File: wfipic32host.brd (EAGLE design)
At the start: 95.2 x 42.9 mm, 47 parts, among them IC1 BMA490L, IC2 TCAN330GD, J1 MLE-105-01-G-DV, J2 MLE-105-01-G-DV, J3 MLE-105-01-G-DV, J4 MLE-105-01-G-DV, U1 PIC32MK0512MCJ048T-I/Y8XTQFP4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, U2 MAX6126B30

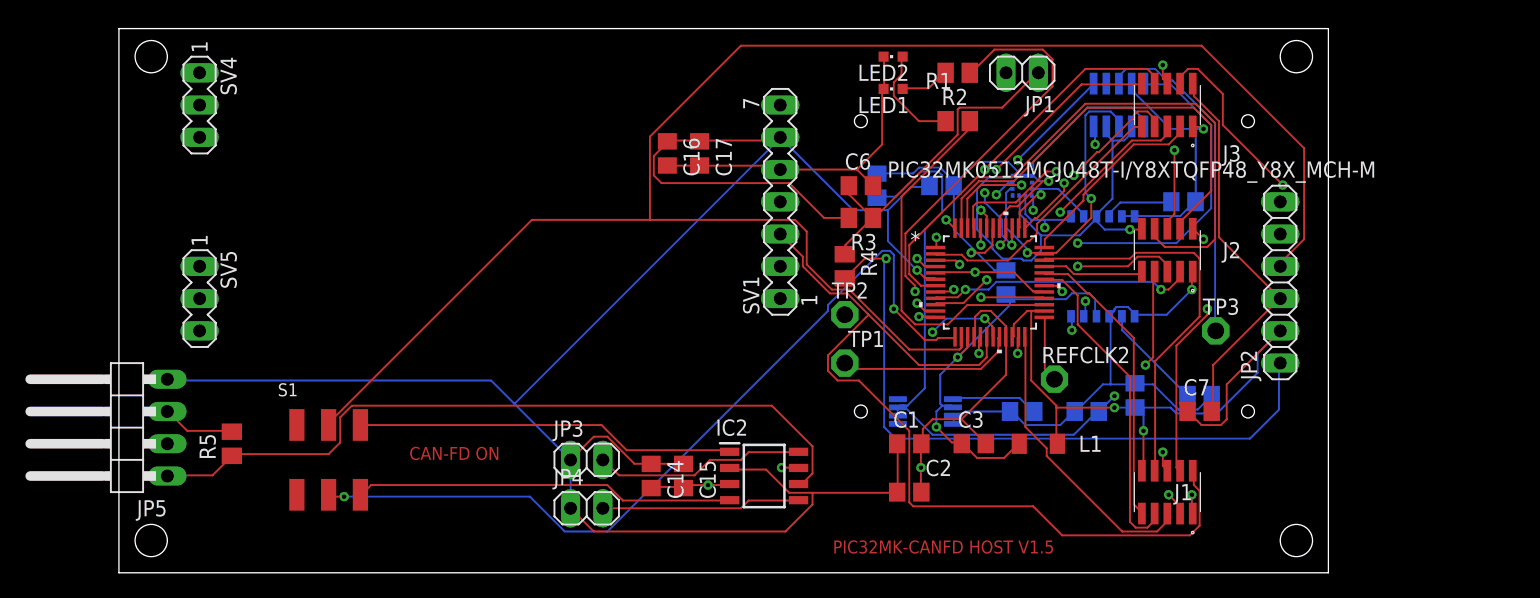
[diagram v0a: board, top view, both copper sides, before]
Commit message: up
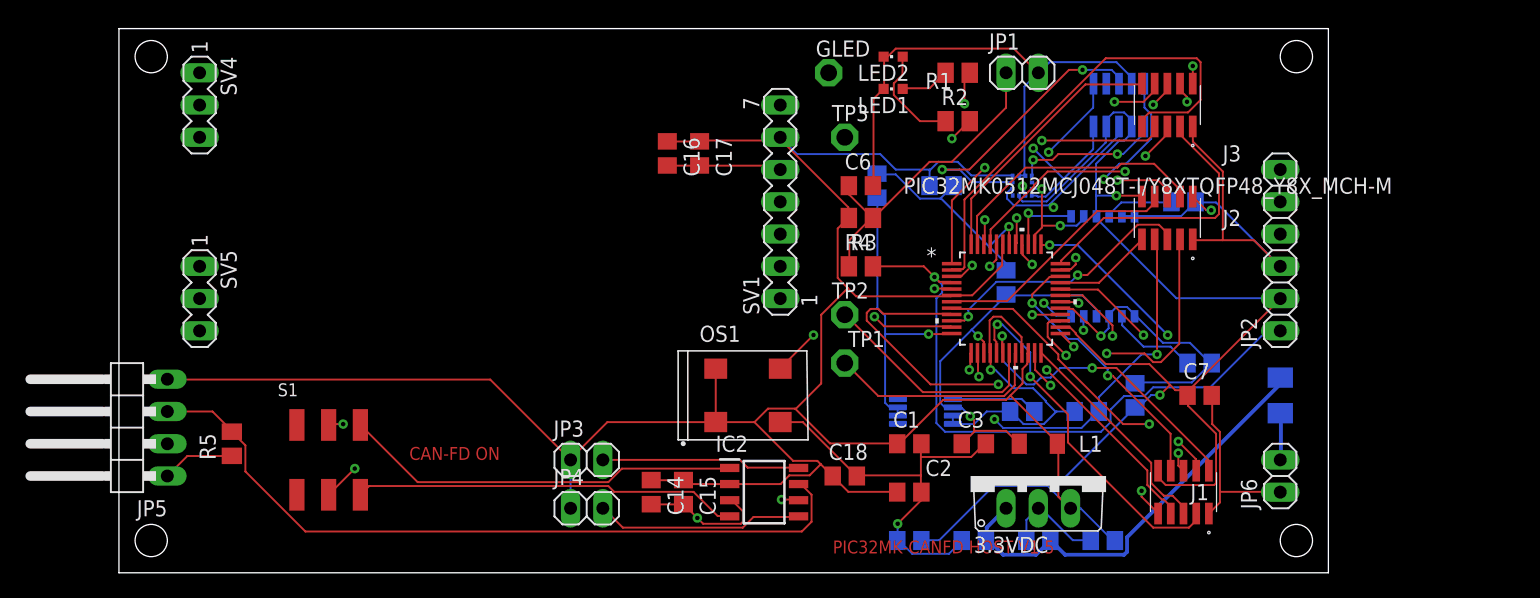
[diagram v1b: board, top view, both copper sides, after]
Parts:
- removed REFCLK2: PTR1PAD1-13, testpad:P1-13
- added 3.3VDC: 3.3 Vreg, linear:TO220V
- added C18, C19, C20: 0.1uf, rcl:C0805
- added C21, C22: 10uf, rcl:C0805
- added GLED: PTR1PAD1-13, testpad:P1-13
- added JP6: DC5+, pinhead:1X02
- added OS1: OSC-OE-CFPS-32, IQD-Frequency-Products:7.2X5.2-4-PAD
- added R6: 0 ohm fuse, rcl:M1206
- moved TP3 32.9 mm to (-1.27, 52.1)
- moved C13 2.54 mm to (26.7, 34.3)
- moved J2 2.54 mm to (24.1, 45.7)
- moved JP2 2.54 mm to (33.0, 43.2)
- moved U1 1.80 mm to (11.4, 39.4)
- moved R4 1.27 mm to (0.00, 41.9), turned to 0 degrees
- moved C14 1.27 mm to (-16.5, 24.1)
- moved C15 1.27 mm to (-14.0, 24.1)
- moved C7 1.27 mm to (26.7, 31.8)
- moved IC2 1.27 mm to (-7.62, 24.1)
- moved J1 1.27 mm to (25.4, 24.1)
- turned JP1 to 0 degrees
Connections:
- removed net N$8: REFCLK2.TP, U1.25
- new net DC_IN: JP6.2, R6.2
- new net DC_INPUT: 3.3VDC.1, C20.1, C21.1, R6.1
- new net OSC_MCU: OS1.3, U1.27
- net GREEN_LED: now also GLED.TP, U1.25; no longer U1.27
- net VDD: now also 3.3VDC.3, C18.1, C19.1, C22.1, OS1.1, OS1.4
- net VSS: now also 3.3VDC.2, C18.2, C19.2, C20.2, C21.2, C22.2, JP6.1, OS1.2
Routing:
- net PGD_C1TX: track 137.8 -> 89.4 mm, vias 0 -> 2
- net DC_INPUT: track 0.00 -> 34.5 mm
- net VSS: track 186.0 -> 220.3 mm
- net EXT_SW2: track 49.2 -> 19.7 mm
- net OSC_MCU: track 0.00 -> 29.3 mm, vias 0 -> 2
- net AN0: track 21.0 -> 44.4 mm
- net PGC_C1RX: track 118.1 -> 95.7 mm
- net U1RX: track 71.4 -> 49.5 mm, vias 0 -> 2
- net VDD: track 285.7 -> 307.0 mm, vias 5 -> 2
- net PWM4ER: track 53.2 -> 35.2 mm
- net PWM1H: track 21.3 -> 38.5 mm
- net SCK2: track 39.7 -> 23.9 mm, vias 2 -> 3
- net BMA_INT2: track 65.8 -> 50.7 mm, vias 2 -> 3
- net RED_LED: track 41.4 -> 26.7 mm
- net INDX2: track 37.1 -> 23.5 mm
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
